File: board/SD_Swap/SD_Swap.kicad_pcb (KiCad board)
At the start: 4 copper layers, 32 x 27 mm, 44 parts, among them J1 USB_C, Q1 Q_Dual_PNP_PNP_E1B1C2E2B2C1, U1 74LVC2G14, U2 RTS5306E, U3 PCB_SD, U4 93AAxxAT, U5 TS3A27518ERTW, U6 SD_SOCKET, U7 AZ1117-3.3, Y1 12MHz

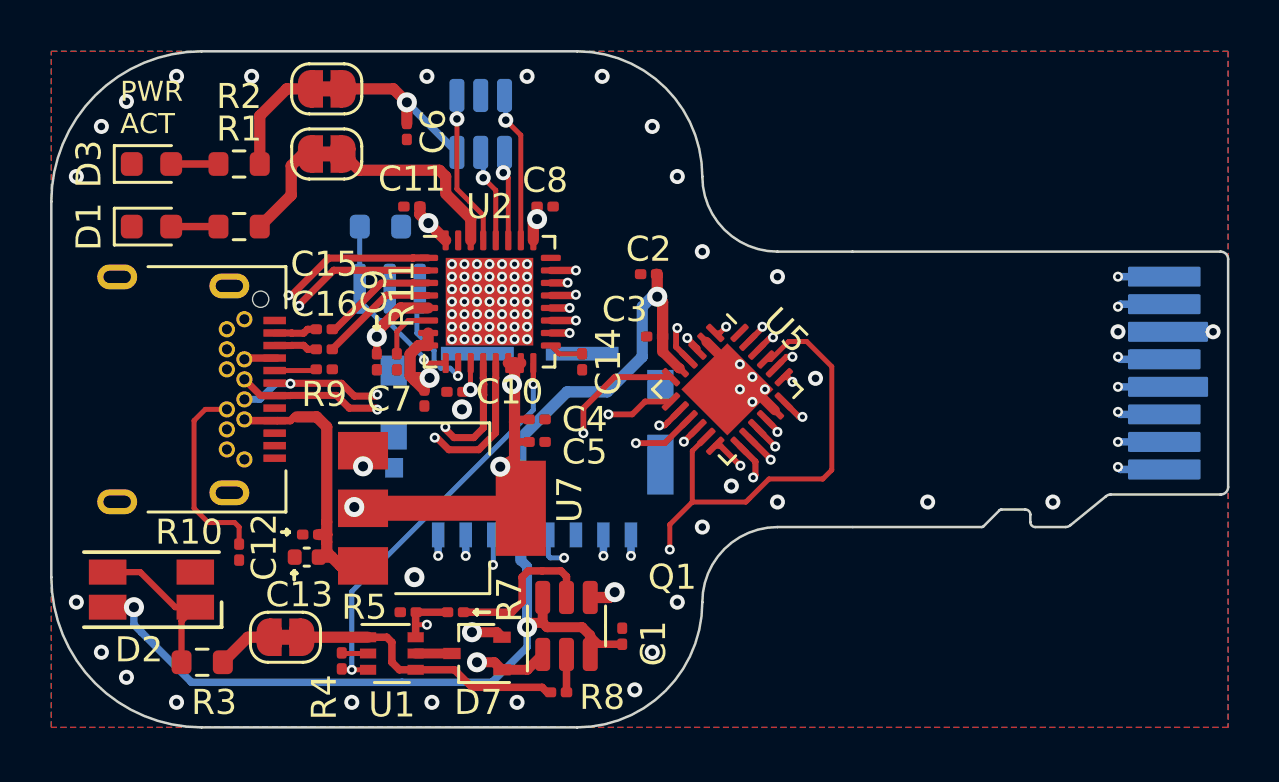
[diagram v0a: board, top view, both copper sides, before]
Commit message: tmp
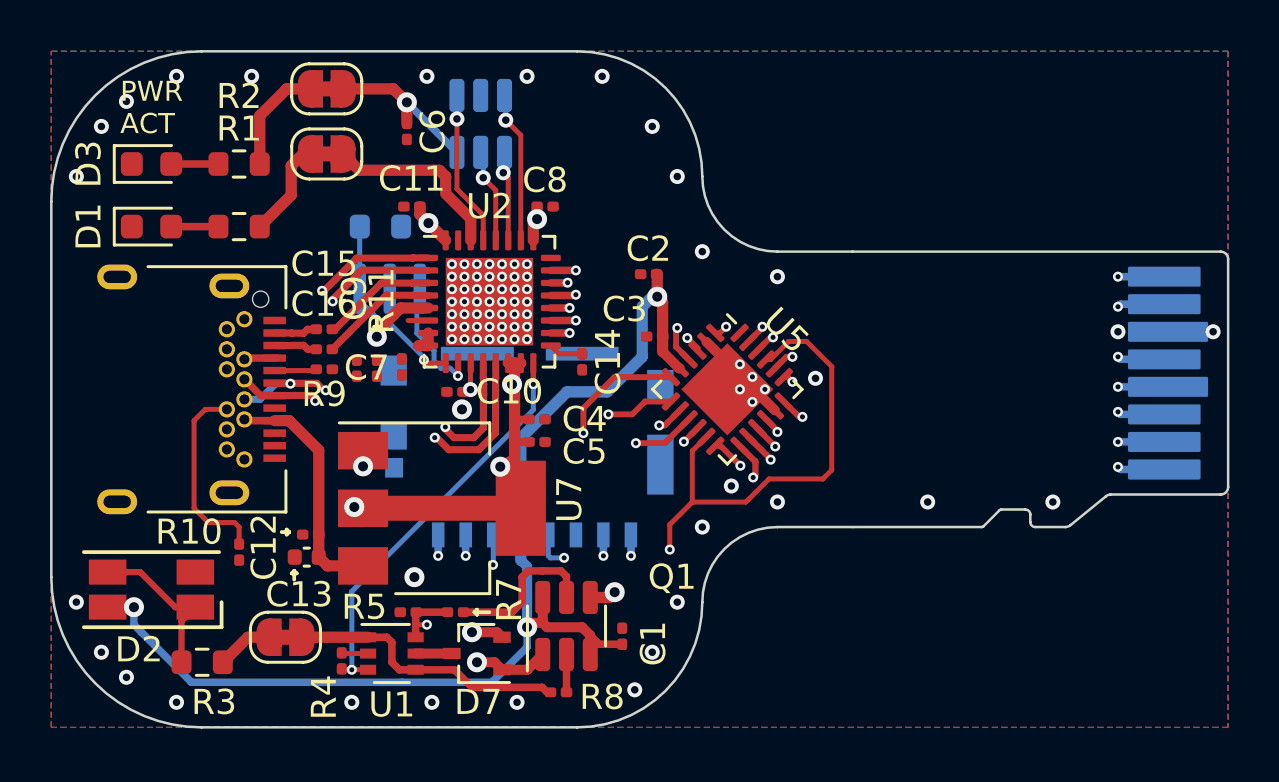
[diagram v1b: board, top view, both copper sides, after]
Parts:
- moved C7 1.54 mm to (105.0, 80.6)
- moved C9 0.84 mm to (103.2, 80.7)
- moved R11 0.84 mm to (104.0, 80.7)
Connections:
- D2 pad 2: VCC -> GND
- D2 pad 3: GND -> Net-(D2-A1)
- D2 pad 4: Net-(D2-A1) -> VCC
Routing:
- net +3.3V: track 28.8 -> 26.0 mm, vias 6 -> 5
- net /USB-: track 17.8 -> 15.9 mm
- net /USB+: track 19.0 -> 17.3 mm
- net Net-(U2-REFF): track 2.32 -> 0.80 mm
- net +5V: track 12.5 -> 11.1 mm
- net +1V2: track 23.4 -> 22.7 mm

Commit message: tmp
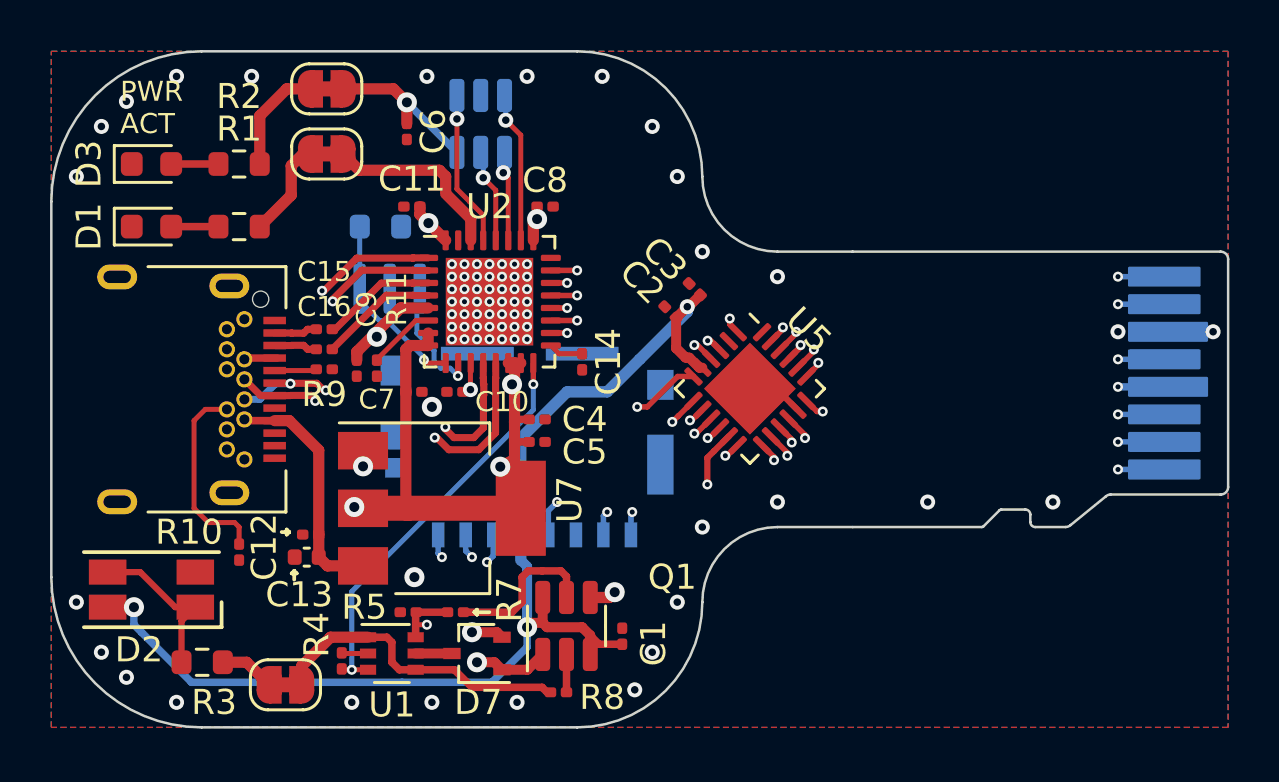
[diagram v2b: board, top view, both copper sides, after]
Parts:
- moved C3 2.48 mm to (116.7, 77.5), turned to 135 degrees
- moved JP3 1.90 mm to (100.3, 93.3)
- moved C2 1.76 mm to (115.7, 78.4), turned to 135 degrees
- moved C7 1.11 mm to (105.5, 81.6), turned to 0 degrees
- moved U5 0.90 mm to (118.9, 81.5)
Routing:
- net +3.3V: track 26.0 -> 32.9 mm
- net Net-(U2-SD_D1): track 13.5 -> 7.67 mm
- net Net-(U5-COM2): track 15.9 -> 10.1 mm
- net /SD_SEL: track 33.7 -> 30.0 mm, vias 2 -> 3
- net Net-(U2-SD_D0): track 12.8 -> 9.40 mm
- net Net-(U5-COM3): track 14.0 -> 10.9 mm
- net Net-(U3-DAT3): track 17.6 -> 15.0 mm
- net Net-(U3-CLK): track 17.6 -> 15.2 mm
- net GND: track 5.56 -> 3.31 mm, vias 87 -> 80
- net Net-(U3-CMD): track 17.6 -> 15.4 mm
- net Net-(U5-COM1): track 13.5 -> 11.4 mm
- net Net-(U2-REFF): track 0.80 -> 2.72 mm
- net Net-(U3-DAT2): track 17.7 -> 15.9 mm
- net Net-(U2-SD_CLK): track 12.9 -> 11.1 mm
- net Net-(U5-COM6): track 14.0 -> 12.5 mm
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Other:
- board text added: "USB3 and 2 are 90ohm diff pair"
- board text added: "{dblquote}(1) Driver Type B Type B driver is the default drive strength, targeted for a fixed impedance distributed system with 50 ohm transmission line, at all available frequencies. Therefore, it is defined as 50 ohm nominal driver. This driver can support total CL of about 15pF for UHS104 card and about 30pF for UHS50 card. Drive strength B is the reference driver for definitions of all the re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"
- board text removed: "UHS50 cards must have 50ohm nominal impedance. There is no length matich requirements but so 0.5mm is ok."
